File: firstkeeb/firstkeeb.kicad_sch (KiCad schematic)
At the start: 2 parts

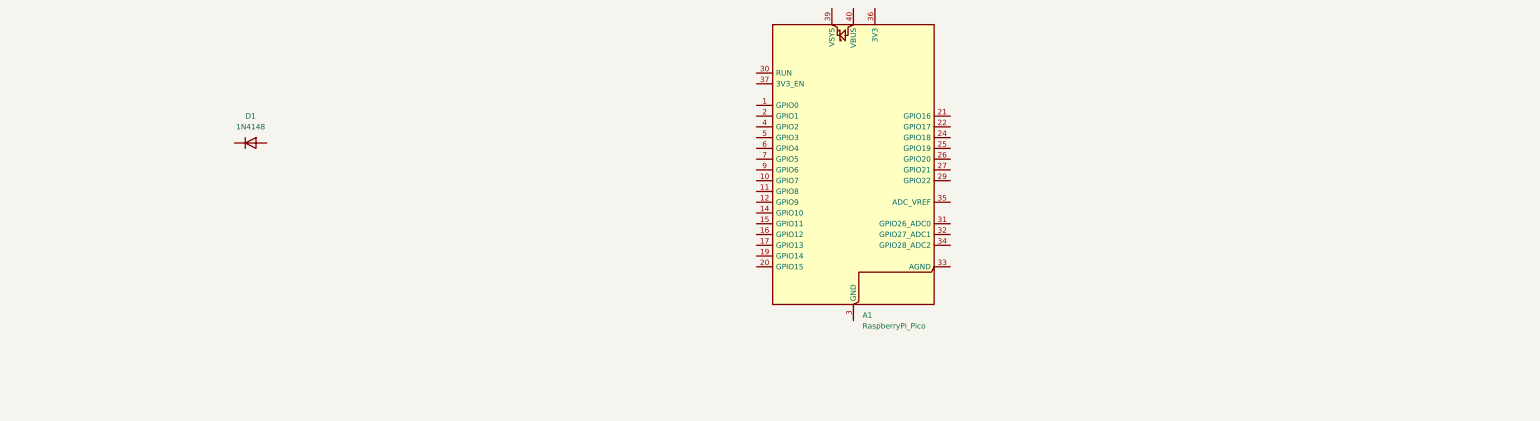
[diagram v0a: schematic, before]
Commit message: okay so far so good its been 1 hours and the half of the keyboard schematic is done
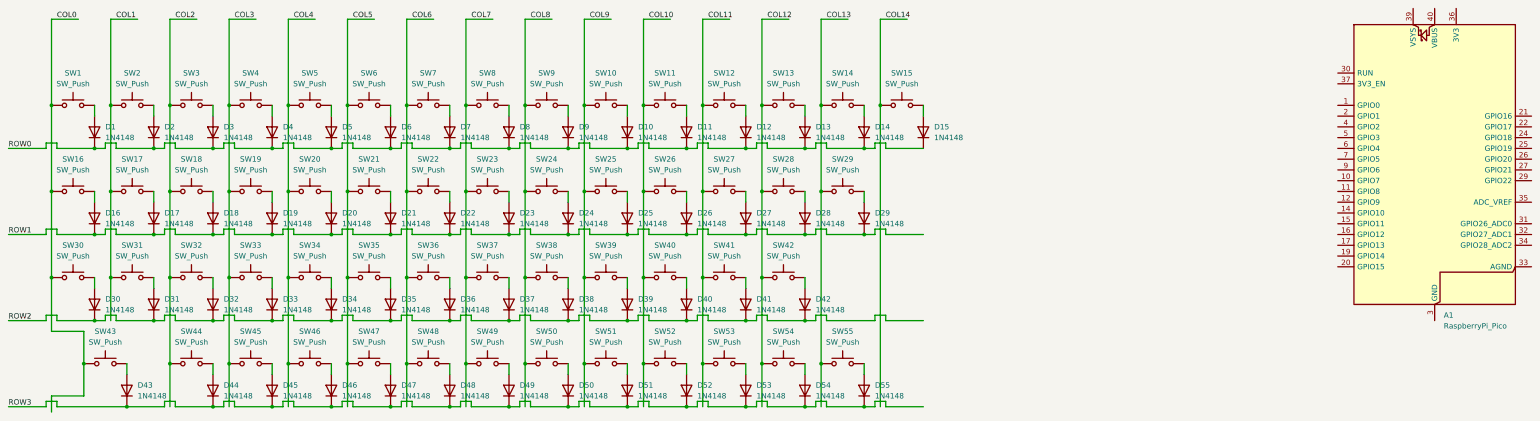
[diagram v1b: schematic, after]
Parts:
- added D10, D11, D12, D13, D14, D15, D16, D17, D18, D19, D2, D20, D21, D22, D23, D24, D25, D26, D27, D28, D29, D3, D30, D31, D32, D33, D34, D35, D36, D37, D38, D39, D4, D40, D41, D42, D43, D44, D45, D46, D47, D48, D49, D5, D50, D51, D52, D53, D54, D55, D6, D7, D8, D9: 1N4148, Diode_THT:D_DO-35_SOD27_P7.62mm_Horizontal, symbol Diode:1N4148
- added SW1, SW10, SW11, SW12, SW13, SW14, SW15, SW16, SW17, SW18, SW19, SW2, SW20, SW21, SW22, SW23, SW24, SW25, SW26, SW27, SW28, SW29, SW3, SW30, SW31, SW32, SW33, SW34, SW35, SW36, SW37, SW38, SW39, SW4, SW40, SW41, SW42, SW43, SW44, SW45, SW46, SW47, SW48, SW49, SW5, SW50, SW51, SW52, SW53, SW54, SW55, SW6, SW7, SW8, SW9: SW_Push, symbol Switch:SW_Push
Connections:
- net ROW0: now reaches D1.1 (K)
- net ROW0: now also D10.1 (K), D11.1 (K), D12.1 (K), D13.1 (K), D14.1 (K), D15.1 (K), D2.1 (K), D3.1 (K), D4.1 (K), D5.1 (K), D6.1 (K), D7.1 (K), D8.1 (K), D9.1 (K)
- net at D1.2 (A): now also SW1.2
- new net: D18.2 (A), SW18.2
- new net: D39.2 (A), SW39.2
- new net: D14.2 (A), SW14.2
- new net: D3.2 (A), SW3.2
- new net: D43.2 (A), SW43.2
- new net: D29.2 (A), SW29.2
- new net: D17.2 (A), SW17.2
- new net: D54.2 (A), SW54.2
- new net: D16.2 (A), SW16.2
- new net: D34.2 (A), SW34.2
- new net: D9.2 (A), SW9.2
- new net: D19.2 (A), SW19.2
- new net: D5.2 (A), SW5.2
- new net: D36.2 (A), SW36.2
- new net: D49.2 (A), SW49.2
- new net: D32.2 (A), SW32.2
- new net: D48.2 (A), SW48.2
- new net: D52.2 (A), SW52.2
- new net: D38.2 (A), SW38.2
- new net: D25.2 (A), SW25.2
- new net: D4.2 (A), SW4.2
- new net: D21.2 (A), SW21.2
- new net: D28.2 (A), SW28.2
- new net: D8.2 (A), SW8.2
- new net: D53.2 (A), SW53.2
- new net: D7.2 (A), SW7.2
- new net: D41.2 (A), SW41.2
- new net: D12.2 (A), SW12.2
- new net: D46.2 (A), SW46.2
- new net: D6.2 (A), SW6.2
- new net: D47.2 (A), SW47.2
- new net: D30.2 (A), SW30.2
- new net: D44.2 (A), SW44.2
- new net: D2.2 (A), SW2.2
- new net: D31.2 (A), SW31.2
- new net: D15.2 (A), SW15.2
- new net: D40.2 (A), SW40.2
- new net: D35.2 (A), SW35.2
- new net: D33.2 (A), SW33.2
- new net: D27.2 (A), SW27.2
- new net: D55.2 (A), SW55.2
- new net: D20.2 (A), SW20.2
- new net: D13.2 (A), SW13.2
- new net: D42.2 (A), SW42.2
- new net: D50.2 (A), SW50.2
- new net: D23.2 (A), SW23.2
- new net: D51.2 (A), SW51.2
- new net: D45.2 (A), SW45.2
- new net: D24.2 (A), SW24.2
- new net: D26.2 (A), SW26.2
- new net: D22.2 (A), SW22.2
- new net: D11.2 (A), SW11.2
- new net: D37.2 (A), SW37.2
- new net: D10.2 (A), SW10.2
- new net COL0: SW1.1, SW16.1, SW30.1, SW43.1
- new net COL1: SW17.1, SW2.1, SW31.1
- new net COL10: SW11.1, SW26.1, SW40.1, SW52.1
- new net COL11: SW12.1, SW27.1, SW41.1, SW53.1
- new net COL12: SW13.1, SW28.1, SW42.1, SW54.1
- new net COL13: SW14.1, SW29.1, SW55.1
- new net COL14: SW15.1
- new net COL2: SW18.1, SW3.1, SW32.1, SW44.1
- new net COL3: SW19.1, SW33.1, SW4.1, SW45.1
- new net COL4: SW20.1, SW34.1, SW46.1, SW5.1
- new net COL5: SW21.1, SW35.1, SW47.1, SW6.1
- new net COL6: SW22.1, SW36.1, SW48.1, SW7.1
- new net COL7: SW23.1, SW37.1, SW49.1, SW8.1
- new net COL8: SW24.1, SW38.1, SW50.1, SW9.1
- new net COL9: SW10.1, SW25.1, SW39.1, SW51.1
- new net ROW1: D16.1 (K), D17.1 (K), D18.1 (K), D19.1 (K), D20.1 (K), D21.1 (K), D22.1 (K), D23.1 (K), D24.1 (K), D25.1 (K), D26.1 (K), D27.1 (K), D28.1 (K), D29.1 (K)
- new net ROW2: D30.1 (K), D31.1 (K), D32.1 (K), D33.1 (K), D34.1 (K), D35.1 (K), D36.1 (K), D37.1 (K), D38.1 (K), D39.1 (K), D40.1 (K), D41.1 (K), D42.1 (K)
- new net ROW3: D43.1 (K), D44.1 (K), D45.1 (K), D46.1 (K), D47.1 (K), D48.1 (K), D49.1 (K), D50.1 (K), D51.1 (K), D52.1 (K), D53.1 (K), D54.1 (K), D55.1 (K)
